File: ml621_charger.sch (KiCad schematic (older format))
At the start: 14 parts, among them J1 USB_B_Micro, Q1 BSS138, U1 ATtiny10-TS, U2 AMS1117-3.3

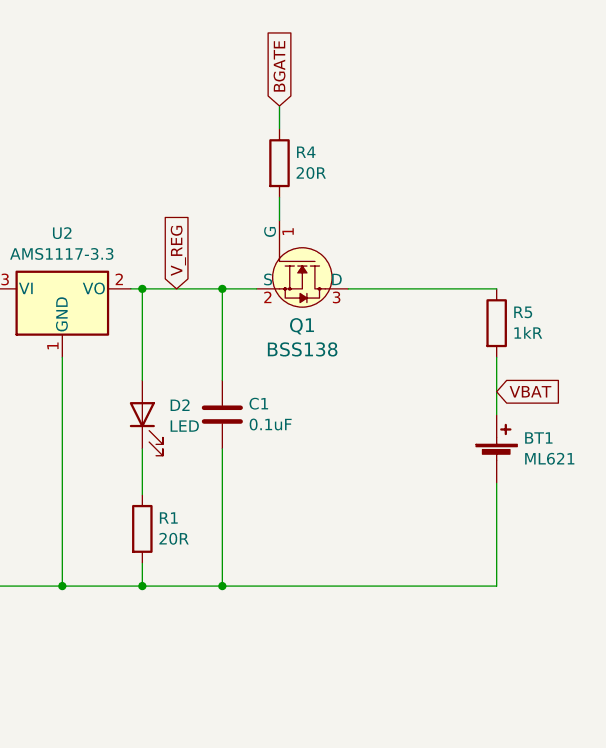
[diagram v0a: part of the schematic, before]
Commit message: Fix charger
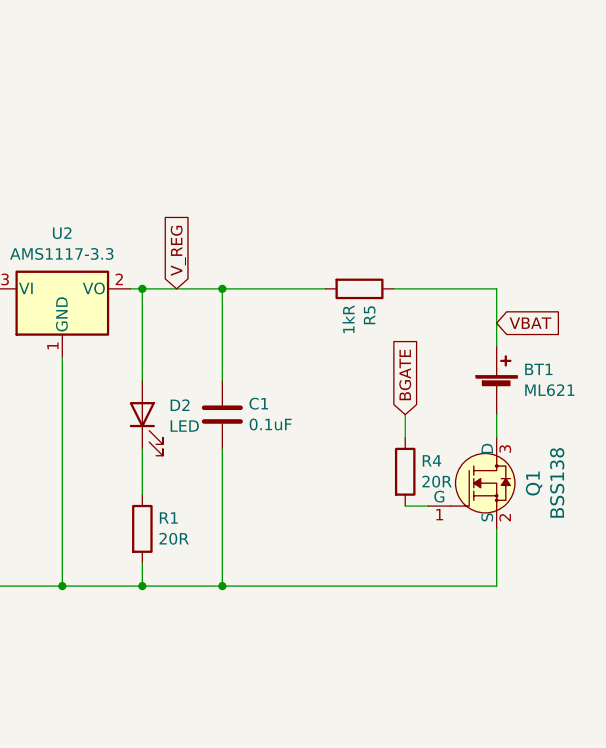
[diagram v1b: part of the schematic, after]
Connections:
- net GNDREF: now also Q1.2 (S); no longer BT1.2 (-)
- net VBAT: now also R5.1; no longer R5.2
- net V_REG: now also R5.2; no longer Q1.2 (S)
- net at Q1.3 (D): now also BT1.2 (-); no longer R5.1
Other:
- moved on the sheet: BT1, Q1, R4, R5
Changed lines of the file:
@@
 EESchema Schematic File Version 4
-LIBS:ml621_charger-cache
-EELAYER 29 0
+EELAYER 30 0
 EELAYER END
 $Descr A4 11693 8268
@@
 L Device:Battery_Cell BT1
 U 1 1 5D7A7B57
-P 4900 2550
-F 0 "BT1" H 5018 2646 50  0000 L CNN
-F 1 "ML621" H 5018 2555 50  0000 L CNN
-F 2 "Battery:BatteryHolder_Keystone_2998_621_6.8x2.2mm" V 4900 2610 50  0001 C CNN
-F 3 "~" V 4900 2610 50  0001 C CNN
-	1    4900 2550
+P 4900 2250
+F 0 "BT1" H 5018 2346 50  0000 L CNN
+F 1 "ML621" H 5018 2255 50  0000 L CNN
+F 2 "Battery:BatteryHolder_Keystone_2998_621_6.8x2.2mm" V 4900 2310 50  0001 C CNN
+F 3 "~" V 4900 2310 50  0001 C CNN
+	1    4900 2250
 	1    0    0    -1
 $EndComp
@@
 Wire Wire Line
 	3700 2500 3700 3100
-Connection ~ 3700 3100
 Wire Wire Line
 	3700 3100 3350 3100
@@
 L dk_Transistors-FETs-MOSFETs-Single:BSS138 Q1
 U 1 1 5ECC513F
-P 4050 1800
-F 0 "Q1" V 4211 1800 60  0000 C CNN
-F 1 "BSS138" V 4317 1800 60  0000 C CNN
-F 2 "digikey-footprints:SOT-23-3" H 4250 2000 60  0001 L CNN
-F 3 "https://www.onsemi.com/pub/Collateral/BSS138-D.PDF" H 4250 2100 60  0001 L CNN
-F 4 "BSS138CT-ND" H 4250 2200 60  0001 L CNN "Digi-Key_PN"
-F 5 "BSS138" H 4250 2300 60  0001 L CNN "MPN"
-F 6 "Discrete Semiconductor Products" H 4250 2400 60  0001 L CNN "Category"
-F 7 "Transistors - FETs, MOSFETs - Single" H 4250 2500 60  0001 L CNN "Family"
-F 8 "https://www.onsemi.com/pub/Collateral/BSS138-D.PDF" H 4250 2600 60  0001 L CNN "DK_Datasheet_Link"
-F 9 "/product-detail/en/on-semiconductor/BSS138/BSS138CT-ND/244294" H 4250 2700 60  0001 L CNN "DK_Detail_Page"
-F 10 "MOSFET N-CH 50V 220MA SOT-23" H 4250 2800 60  0001 L CNN "Description"
-F 11 "ON Semiconductor" H 4250 2900 60  0001 L CNN "Manufacturer"
-F 12 "Active" H 4250 3000 60  0001 L CNN "Status"
-	1    4050 1800
-	0    1    1    0
+P 4900 2650
+F 0 "Q1" V 5061 2650 60  0000 C CNN
+F 1 "BSS138" V 5167 2650 60  0000 C CNN
+F 2 "digikey-footprints:SOT-23-3" H 5100 2850 60  0001 L CNN
+F 3 "https://www.onsemi.com/pub/Collateral/BSS138-D.PDF" H 5100 2950 60  0001 L CNN
+F 4 "BSS138CT-ND" H 5100 3050 60  0001 L CNN "Digi-Key_PN"
+F 5 "BSS138" H 5100 3150 60  0001 L CNN "MPN"
+F 6 "Discrete Semiconductor Products" H 5100 3250 60  0001 L CNN "Category"
+F 7 "Transistors - FETs, MOSFETs - Single" H 5100 3350 60  0001 L CNN "Family"
+F 8 "https://www.onsemi.com/pub/Collateral/BSS138-D.PDF" H 5100 3450 60  0001 L CNN "DK_Datasheet_Link"
+F 9 "/product-detail/en/on-semiconductor/BSS138/BSS138CT-ND/244294" H 5100 3550 60  0001 L CNN "DK_Detail_Page"
+F 10 "MOSFET N-CH 50V 220MA SOT-23" H 5100 3650 60  0001 L CNN "Description"
+F 11 "ON Semiconductor" H 5100 3750 60  0001 L CNN "Manufacturer"
+F 12 "Active" H 5100 3850 60  0001 L CNN "Status"
+	1    4900 2650
+	1    0    0    -1
 $EndComp
 $Comp
 L Device:R R5
 U 1 1 5ECC848D
-P 4900 1950
-F 0 "R5" H 4970 1996 50  0000 L CNN
-F 1 "1kR" H 4970 1905 50  0000 L CNN
-F 2 "Resistor_SMD:R_0805_2012Metric" V 4830 1950 50  0001 C CNN
-F 3 "~" H 4900 1950 50  0001 C CNN
-	1    4900 1950
-	1    0    0    -1
+P 4300 1800
+F 0 "R5" H 4370 1846 50  0000 L CNN
+F 1 "1kR" H 4370 1755 50  0000 L CNN
+F 2 "Resistor_SMD:R_0805_2012Metric" V 4230 1800 50  0001 C CNN
+F 3 "~" H 4300 1800 50  0001 C CNN
+	1    4300 1800
+	0    1    1    0
 $EndComp
 Wire Wire Line
 	3350 1800 3700 1800
 Wire Wire Line
-	4900 3100 4900 2650
-Wire Wire Line
-	3700 3100 4900 3100
-Wire Wire Line
-	4900 2350 4900 2100
-Wire Wire Line
-	4900 1800 4250 1800
-Wire Wire Line
-	3850 1800 3700 1800
-Connection ~ 3700 1800
+	4900 2050 4900 1800
 $Comp
 L Device:R R3
@@
 	0    1    1    0
 $EndComp
-Text GLabel 4900 2250 2    50   Input ~ 0
+Text GLabel 4900 1950 2    50   Input ~ 0
 VBAT
 Text GLabel 2700 4150 1    50   Input ~ 0
@@
 Wire Wire Line
 	3500 4650 3300 4650
-Text GLabel 3950 1000 1    50   Input ~ 0
+Text GLabel 4500 2350 1    50   Input ~ 0
 BGATE
 Wire Wire Line
-	3950 1400 3950 1500
+	4500 2750 4600 2750
 Text GLabel 3500 4550 2    50   Input ~ 0
 BGATE
@@
 L Device:R R4
 U 1 1 5ECE28A8
-P 3950 1250
-F 0 "R4" H 4020 1296 50  0000 L CNN
-F 1 "20R" H 4020 1205 50  0000 L CNN
-F 2 "Resistor_SMD:R_0805_2012Metric" V 3880 1250 50  0001 C CNN
-F 3 "~" H 3950 1250 50  0001 C CNN
-	1    3950 1250
-	1    0    0    -1
-$EndComp
-Wire Wire Line
-	3950 1000 3950 1100
+P 4500 2600
+F 0 "R4" H 4570 2646 50  0000 L CNN
+F 1 "20R" H 4570 2555 50  0000 L CNN
+F 2 "Resistor_SMD:R_0805_2012Metric" V 4430 2600 50  0001 C CNN
+F 3 "~" H 4500 2600 50  0001 C CNN
+	1    4500 2600
+	1    0    0    -1
+$EndComp
+Wire Wire Line
+	4500 2350 4500 2450
 Wire Wire Line
 	4150 4750 4250 4750
+Wire Wire Line
+	3700 1800 4150 1800
+Connection ~ 3700 1800
+Wire Wire Line
+	4900 1800 4450 1800
+Wire Wire Line
+	4900 2350 4900 2450
+Wire Wire Line
+	4900 2850 4900 3100
+Wire Wire Line
+	4900 3100 3700 3100
+Connection ~ 3700 3100
 $EndSCHEMATC
